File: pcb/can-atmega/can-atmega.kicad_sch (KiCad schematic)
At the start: 25 parts, among them J1 Screw_Terminal_01x05, J3 Conn_02x03_Odd_Even, J4 Connector_female, U1 LM1117-5.0, U2 TJA1051T, U3 MCP2515-xSO, U4 ATmega328P-A, X1 16MHz, X2 16MHz

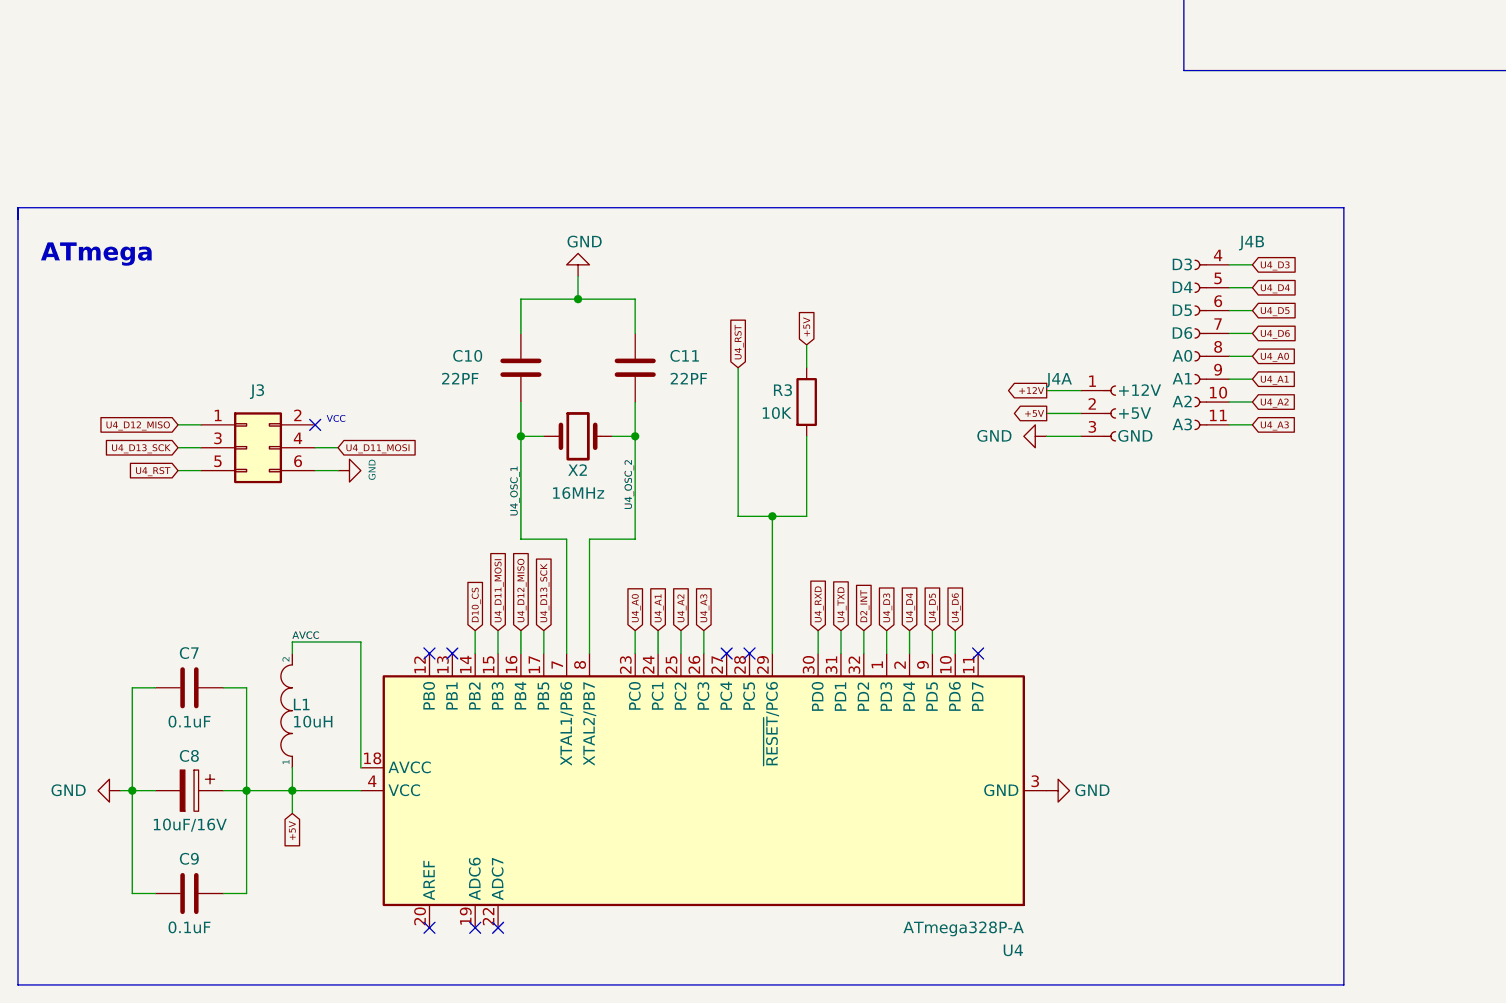
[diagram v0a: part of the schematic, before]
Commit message: pcb update
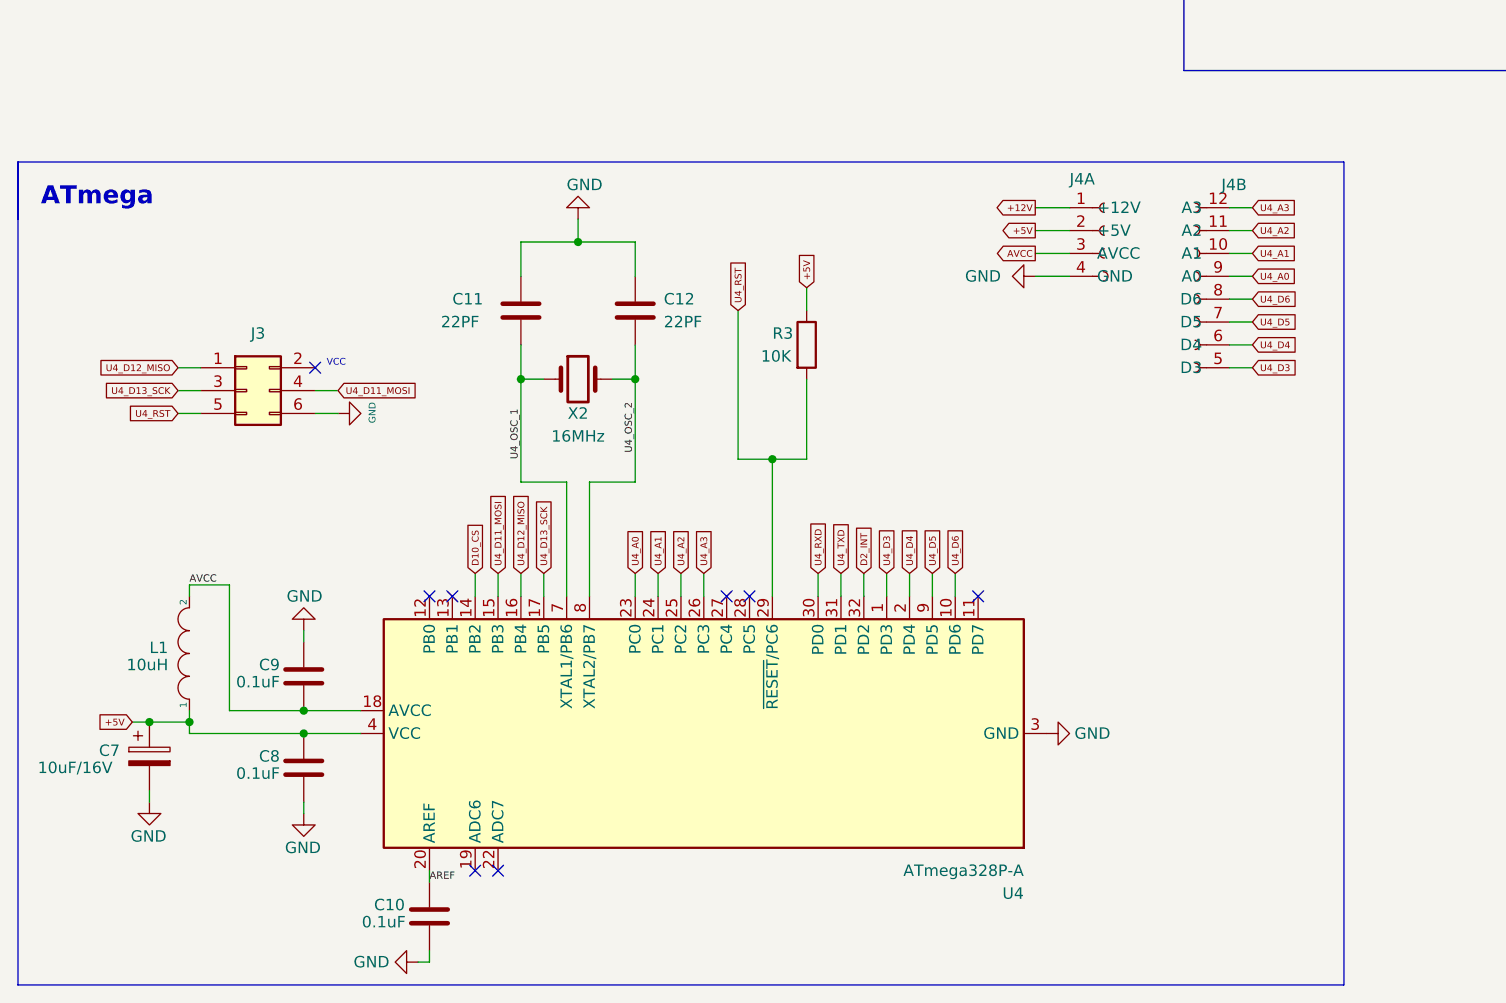
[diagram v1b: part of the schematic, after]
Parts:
- removed J4: Connector_female, CAN_ATmega:Connector_female, symbol CAN_ATmega:Connector_female
- added C10: 0.1uF, Capacitor_SMD:C_1206_3216Metric, symbol Device:C
- added J4: Connector_female_4x8, CAN_ATmega:Connector_female_4x8, symbol CAN_ATmega:Connector_female_4x8
- L1: footprint Inductor_SMD:L_0805_2012Metric -> Inductor_SMD:L_Neosid_SMS-ME3010
- LED1: footprint LED_SMD:LED_0805_2012Metric -> led_tube_MEN_12711000:led_tube_MEN_12711000
- renumbered C10 to C11, C11 to C12, C8 to C7, C9 to C8, C7 to C9
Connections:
- net +12V: now also J4.1 (+12V)
- net +5V: now also J4.2 (+5V); no longer C9.1
- net AVCC: now also C9.2, J4.3 (AVCC)
- net GND: now also C9.1, C10.1, J4.4 (GND); no longer C9.2
- net U4_A0: now also J4.9 (A0)
- net U4_A1: now also J4.10 (A1)
- net U4_A2: now also J4.11 (A2)
- net U4_A3: now also J4.12 (A3)
- net U4_D3: now also J4.5 (D3)
- net U4_D4: now also J4.6 (D4)
- net U4_D5: now also J4.7 (D5)
- net U4_D6: now also J4.8 (D6)
- net AREF: now reaches U4.20 (AREF)
- net AREF: now also C10.2
- no-connect marks 16 -> 15
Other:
- moved on the sheet: C11, C12, C7, C8, C9, J3, L1, R3, U4, X2

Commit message: pcb fab 2025-07-04
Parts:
- C2, C7: footprint Capacitor_SMD:C_1206_3216Metric -> Capacitor_Tantalum_SMD:CP_EIA-3216-18_Kemet-A
- LED1: footprint led_tube_MEN_12711000:led_tube_MEN_12711000 -> LED_SMD:LED_0805_2012Metric
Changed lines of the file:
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@@
     (property "Reference" "C7" (id 0) (at 24.13 169.545 0))
     (property "Value" "10uF/16V" (id 1) (at 20.32 171.45 0))
-    (property "Footprint" "Capacitor_SMD:C_1206_3216Metric" (id 2) (at 29.5402 173.99 0)
+    (property "Footprint" "Capacitor_Tantalum_SMD:CP_EIA-3216-18_Kemet-A" (id 2) (at 29.5402 173.99 0)
       (effects (font (size 1.27 1.27)) hide)
     )
@@
       (effects (font (size 1.27 1.27)) (justify left))
     )
-    (property "Footprint" "Capacitor_SMD:C_1206_3216Metric" (id 2) (at 238.4552 78.74 0)
+    (property "Footprint" "Capacitor_Tantalum_SMD:CP_EIA-3216-18_Kemet-A" (id 2) (at 238.4552 78.74 0)
       (effects (font (size 1.27 1.27)) hide)
     )
@@
       (effects (font (size 1.27 1.27)) (justify right))
     )
-    (property "Footprint" "led_tube_MEN_12711000:led_tube_MEN_12711000" (id 2) (at 68.58 38.1 0)
+    (property "Footprint" "LED_SMD:LED_0805_2012Metric" (id 2) (at 68.58 38.1 0)
       (effects (font (size 1.27 1.27)) hide)
     )
@@
     )
     (path "/bb2e7277-c4e4-4107-b435-483d93c0988e"
-      (reference "C2") (unit 1) (value "10uF/16V") (footprint "Capacitor_SMD:C_1206_3216Metric")
+      (reference "C2") (unit 1) (value "10uF/16V") (footprint "Capacitor_Tantalum_SMD:CP_EIA-3216-18_Kemet-A")
     )
     (path "/d3f71e8a-9a2f-4a97-9998-c927aa032ae4"
@@
     )
     (path "/3d9a1a36-2f4f-43b7-9e0d-58b9f0e71e07"
-      (reference "C7") (unit 1) (value "10uF/16V") (footprint "Capacitor_SMD:C_1206_3216Metric")
+      (reference "C7") (unit 1) (value "10uF/16V") (footprint "Capacitor_Tantalum_SMD:CP_EIA-3216-18_Kemet-A")
     )
     (path "/86084dcb-9556-40bb-a19f-7ff0d38f31a7"
@@
     )
     (path "/cb986dfa-de7c-4747-ad08-78d0c57370f5"
-      (reference "LED1") (unit 1) (value "Green") (footprint "led_tube_MEN_12711000:led_tube_MEN_12711000")
+      (reference "LED1") (unit 1) (value "Green") (footprint "LED_SMD:LED_0805_2012Metric")
     )
     (path "/8ef730e6-7745-407b-b999-e674f4f34f5f"
